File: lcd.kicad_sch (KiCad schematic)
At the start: 2 parts, among them J1 687110149022, J2 687140149022

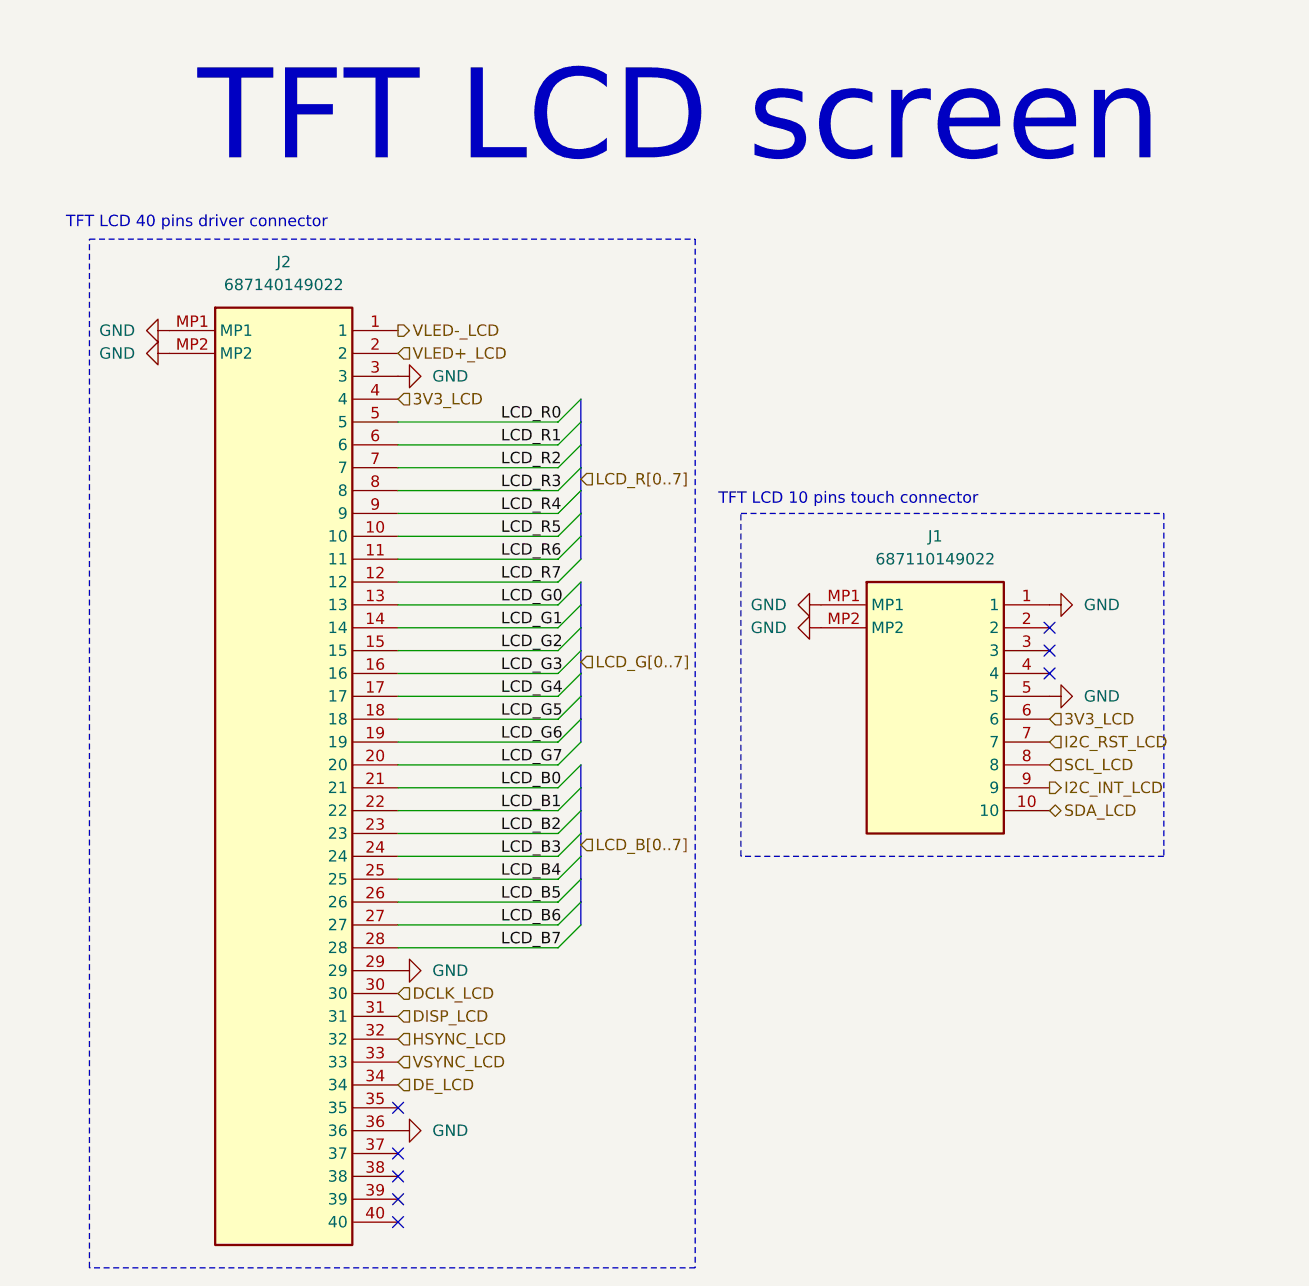
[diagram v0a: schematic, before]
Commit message: Continue schematic review
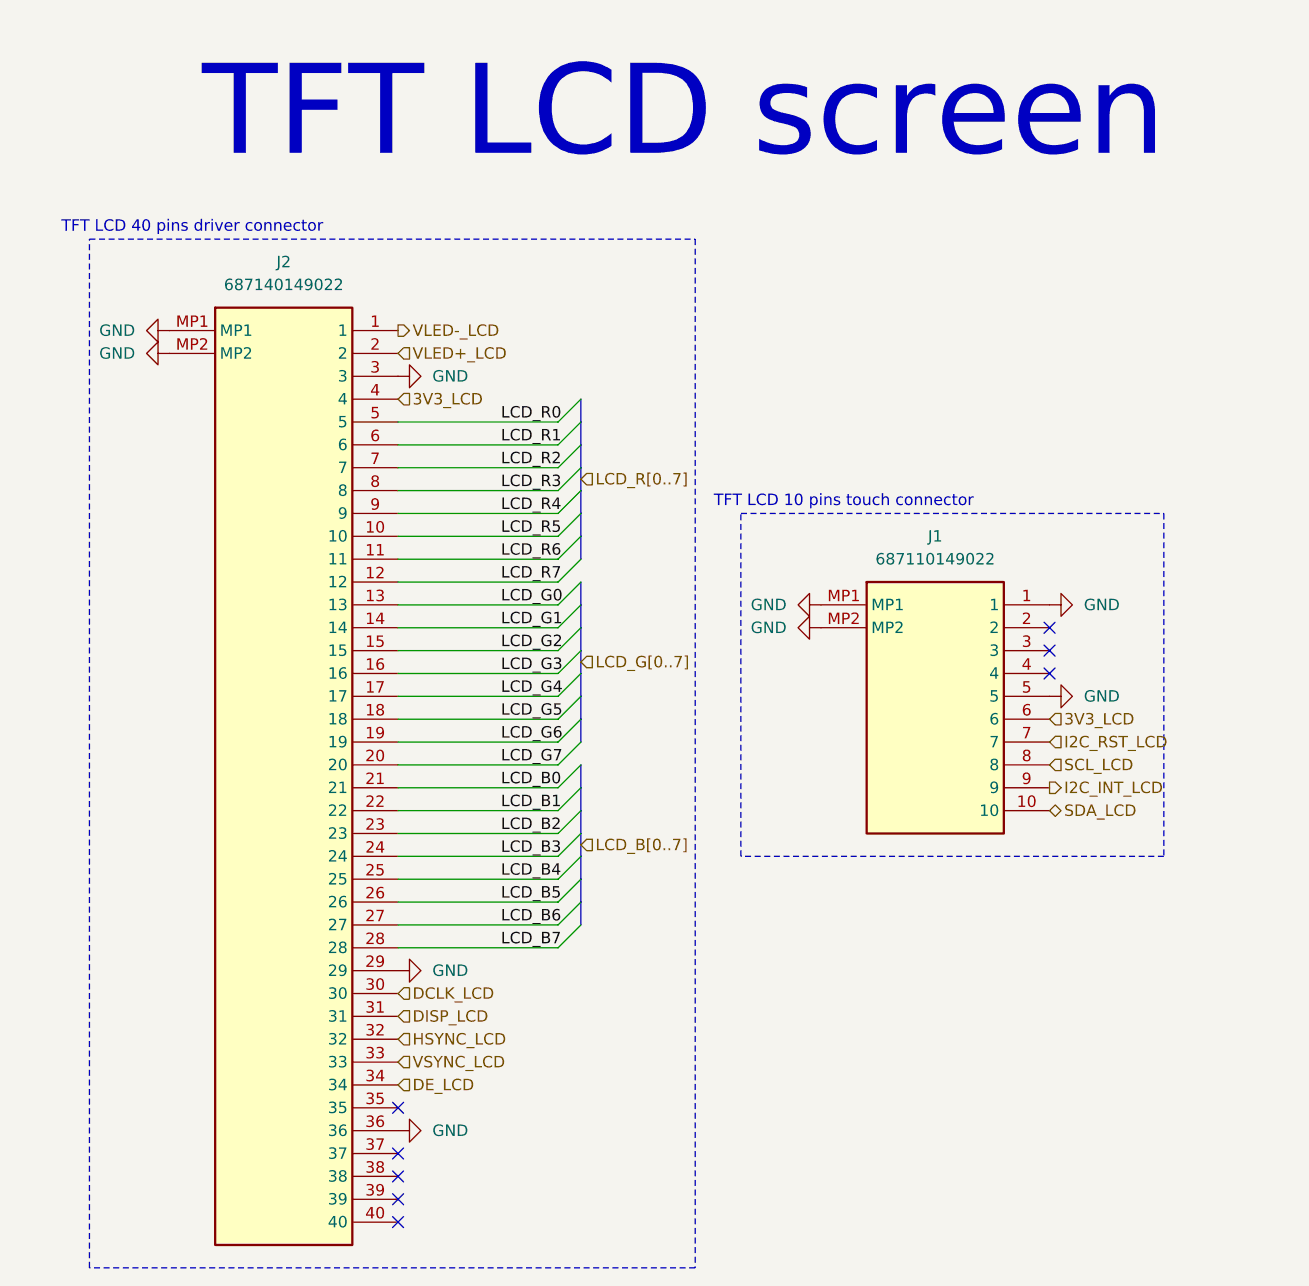
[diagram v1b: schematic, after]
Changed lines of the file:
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@@
 	(text "TFT LCD 40 pins driver connector"
 		(exclude_from_sim no)
-		(at 95.758 36.322 0)
+		(at 95.25 36.83 0)
 		(effects
 			(font
@@
 	(text "TFT LCD 10 pins touch connector"
 		(exclude_from_sim no)
-		(at 168.148 67.056 0)
+		(at 167.64 67.31 0)
 		(effects
 			(font
@@
 	(text "TFT LCD screen"
 		(exclude_from_sim no)
-		(at 149.352 24.638 0)
+		(at 149.86 24.13 0)
 		(effects
 			(font
